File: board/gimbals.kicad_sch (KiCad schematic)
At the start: 4 parts

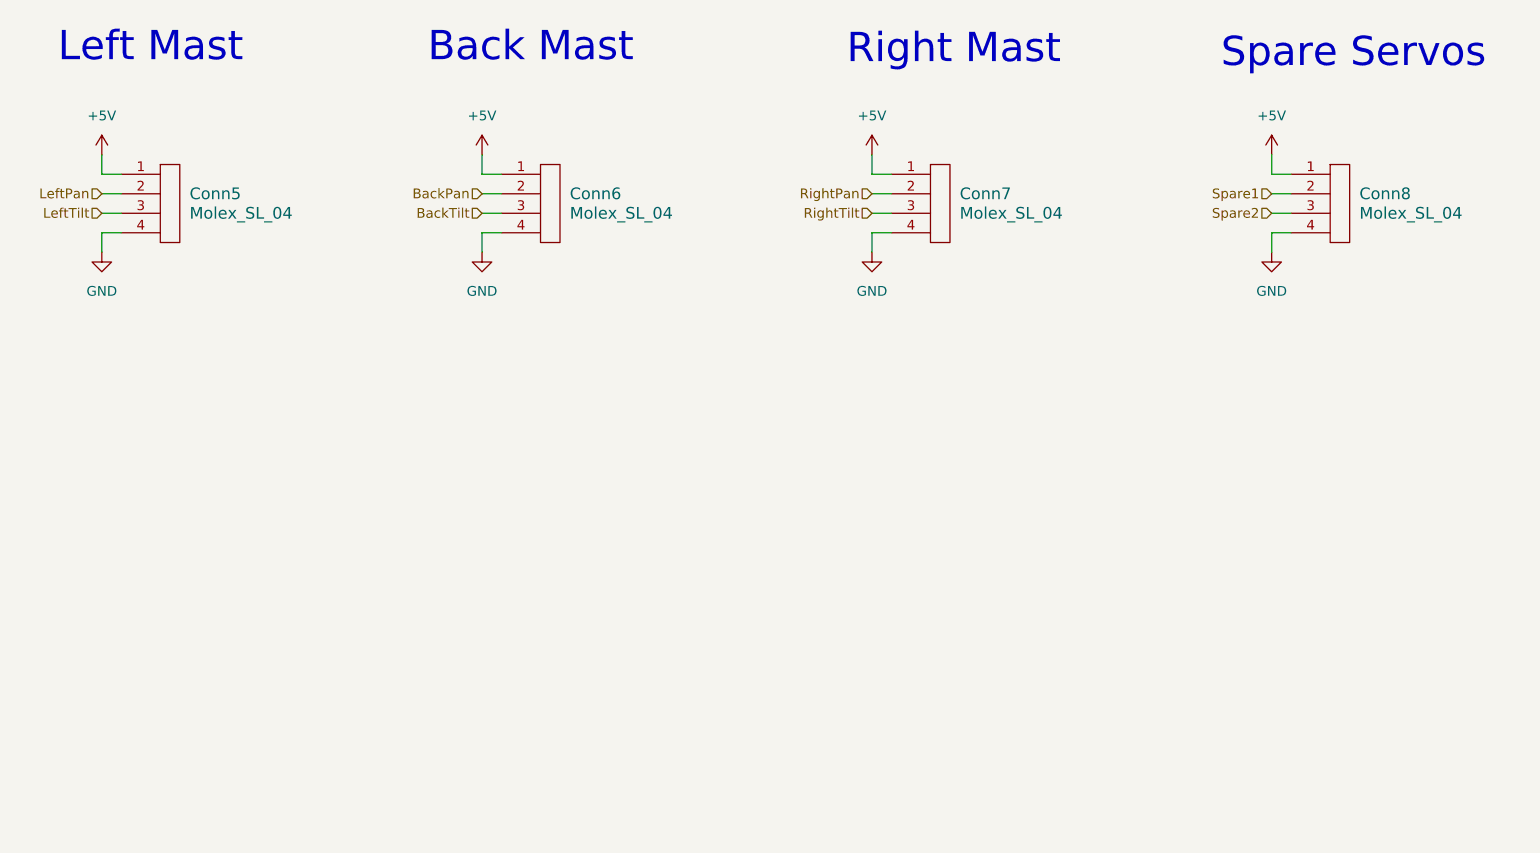
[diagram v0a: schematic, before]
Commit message: Preliminary changes for rev2
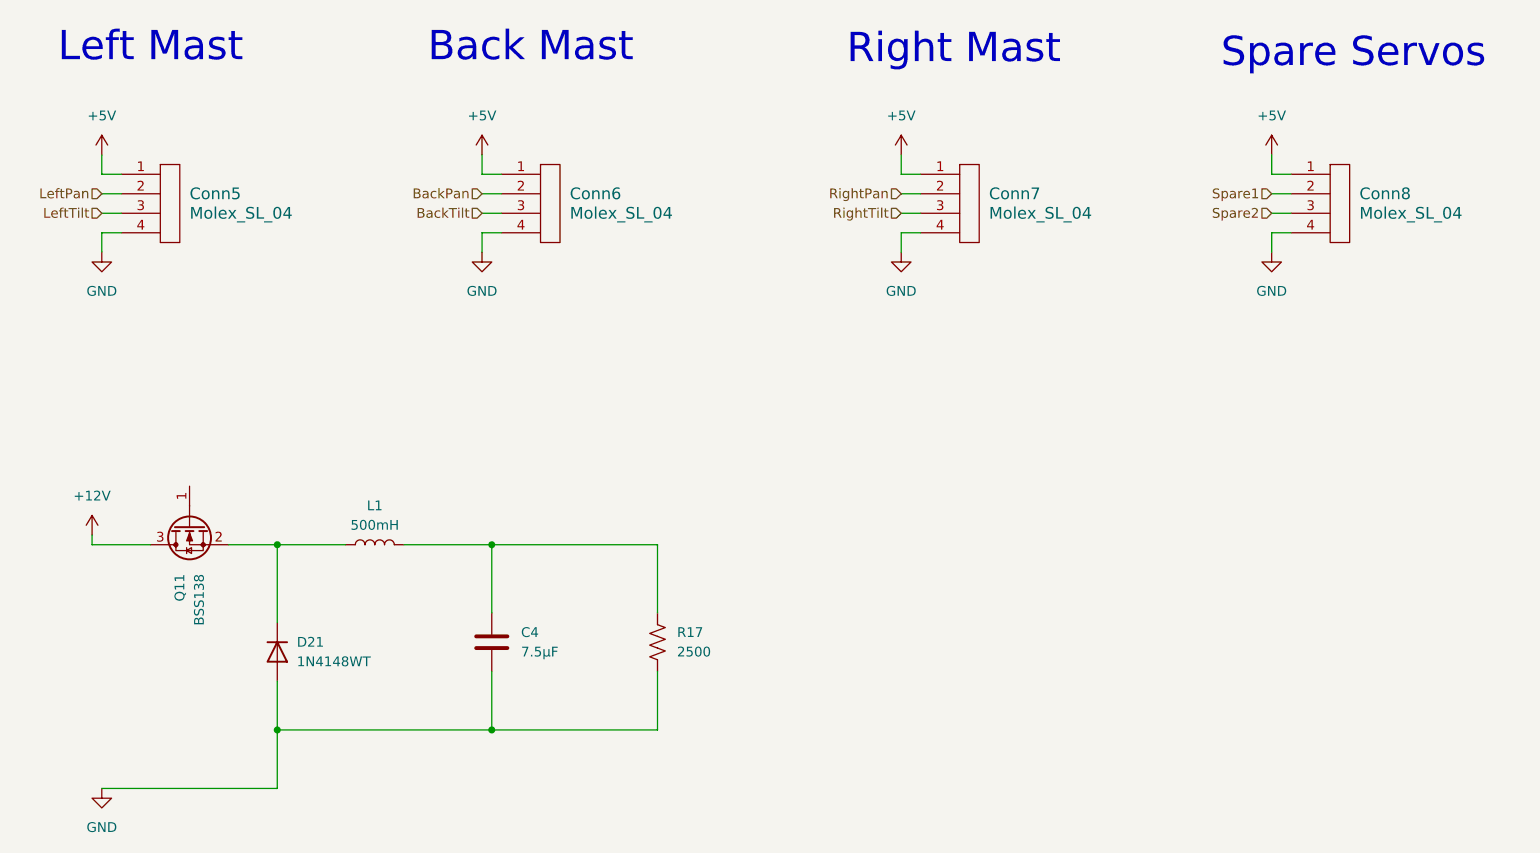
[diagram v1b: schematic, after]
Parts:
- added C4: 7.5µF, Capacitor_SMD:C_0603_1608Metric_Pad1.08x0.95mm_HandSolder, symbol Device:C
- added D21: 1N4148WT, Diode_SMD:D_SOD-523, symbol Diode:1N4148WT
- added L1: 500mH, symbol Device:L
- added Q11: BSS138, Package_TO_SOT_SMD:SOT-23, symbol Transistor_FET:BSS138
- added R17: 2500, Resistor_SMD:R_0603_1608Metric_Pad0.98x0.95mm_HandSolder, symbol Device:R_US
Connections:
- net GND: now also C4.2, D21.2 (A), R17.2
- new net: C4.1, L1.2, R17.1
- new net: D21.1 (K), L1.1, Q11.2 (S)
- new net +12V: Q11.3 (D)
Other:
- moved on the sheet: Conn7
